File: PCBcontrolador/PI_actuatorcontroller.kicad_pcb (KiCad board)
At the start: 2 copper layers, 95.7 x 60 mm, 43 parts, among them IC1 TLV9032QDGKRQ1, J1 ACTUATOR1, J3 Barrel_Jack_Switch, U1 INA381A1IDSGR

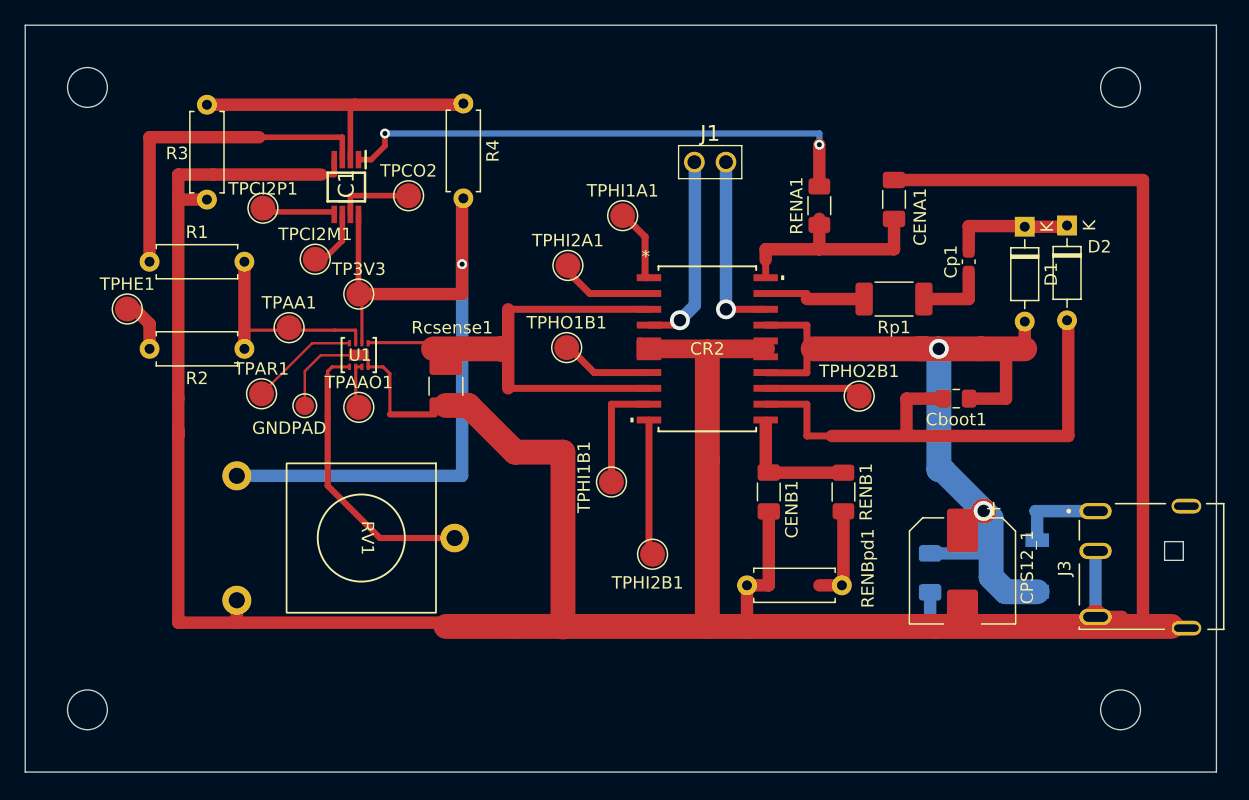
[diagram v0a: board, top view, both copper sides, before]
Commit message: PCB controller final version
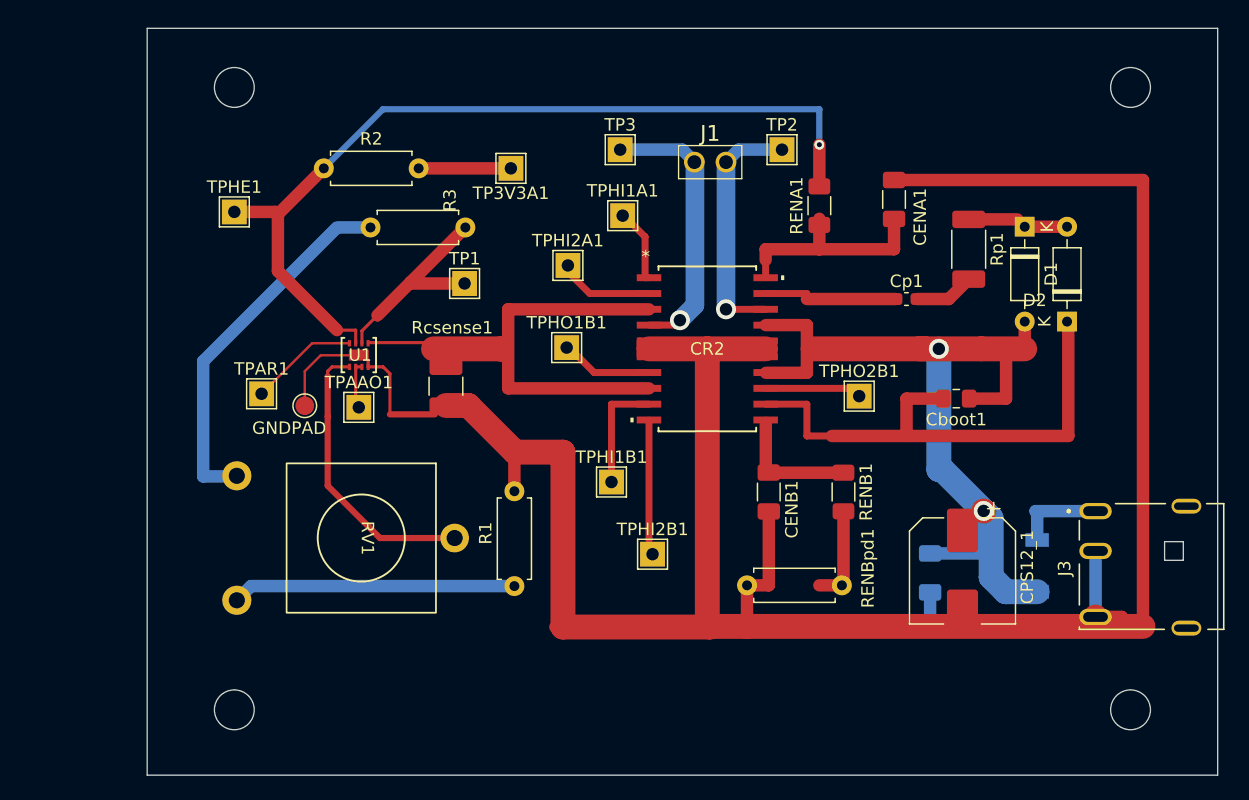
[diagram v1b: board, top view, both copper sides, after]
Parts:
- removed IC1: TLV9032QDGKRQ1, TLV9032QDGKRQ1:SOP65P490X110-8N
- removed R4: 2k, Resistor_THT:R_Axial_DIN0207_L6.3mm_D2.5mm_P7.62mm_Horizontal
- removed TP3V3, TPAA1, TPCI2M1, TPCI2P1, TPCO2: TestPoint, TestPoint:TestPoint_Pad_D2.0mm
- added TP1: TestPoint, TestPoint:TestPoint_THTPad_2.0x2.0mm_Drill1.0mm, F.Cu at (134.5, 81.8)
- added TP2: TestPoint, TestPoint:TestPoint_THTPad_2.0x2.0mm_Drill1.0mm, F.Cu at (160.0, 71.0)
- added TP3: TestPoint, TestPoint:TestPoint_THTPad_2.0x2.0mm_Drill1.0mm, F.Cu at (147.0, 71.0)
- added TP3V3A1: TestPoint, TestPoint:TestPoint_THTPad_2.0x2.0mm_Drill1.0mm, F.Cu at (138.2, 72.5)
- R1, R3: value 2k -> 10K
- R2: value 2k -> 10k
- TPAAO1, TPAR1, TPHE1, TPHI1A1, TPHI1B1, TPHI2A1, TPHI2B1, TPHO1B1, TPHO2B1: footprint TestPoint:TestPoint_Pad_D2.0mm -> TestPoint:TestPoint_THTPad_2.0x2.0mm_Drill1.0mm
- moved R1 39.2 mm to (138.5, 106.1), turned to 90 degrees
- moved R3 20.9 mm to (134.6, 77.2), turned to 180 degrees
- moved R2 15.8 mm to (123.2, 72.5), turned to 0 degrees
- moved REF** 11.8 mm to (116.0, 66.0)
- moved REF** 11.8 mm to (116.0, 115.9)
- moved TPHE1 11.6 mm to (116.0, 76.0)
- moved D2 7.72 mm to (182.9, 84.8), turned to 90 degrees
- moved Rp1 7.21 mm to (175.0, 79.0), turned to -90 degrees
- moved Cp1 5.83 mm to (170.0, 83.0), turned to 0 degrees
- moved REF** 0.80 mm to (188.0, 116.0)
- moved REF** 0.80 mm to (188.0, 66.0)
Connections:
- Cp1 pad 1: Net-(Cp1-Pad1) -> Net-(CR2-VCP)
- Cp1 pad 2: Net-(D1-K) -> Net-(Cp1-Pad2)
- D2 pad 1: Net-(D1-K) -> Net-(CR2-VBOOT)
- D2 pad 2: Net-(CR2-VBOOT) -> Net-(D1-K)
- GNDPAD pad 1: (no net) -> GND
- R1 pad 1: /EnA_soft -> Net-(R1-Pad1)
- R1 pad 2: /calert -> GND
- R2 pad 1: /calert -> /GPIO enable
- R2 pad 2: /GPIO enable -> Net-(R2-Pad2)
- R3 pad 1: GND -> +3V3
- R3 pad 2: Net-(IC1-IN1-) -> Net-(R3-Pad2)
- RENA1 pad 2: /EnA_buf -> /GPIO enable
- RV1 pad 1: +3V3 -> Net-(R3-Pad2)
- RV1 pad 3: GND -> Net-(R1-Pad1)
- Rp1 pad 1: Net-(Cp1-Pad1) -> Net-(D1-K)
- Rp1 pad 2: Net-(CR2-VCP) -> Net-(Cp1-Pad2)
- U1 pad 3: /calert -> /GPIO enable
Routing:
- net GND: track 309.0 -> 225.2 mm
- net /GPIO enable: track 3.98 -> 71.7 mm, vias 0 -> 1
- net +3V3: track 61.2 -> 17.6 mm, vias 1 -> 0
- net /EnA_buf: track 43.6 -> 0.00 mm, vias 2 -> 0
- net Net-(R3-Pad2): track 0.00 -> 29.3 mm
- net /EnA_soft: track 27.3 -> 0.00 mm
- net Net-(IC1-IN1-): track 25.2 -> 0.00 mm
- net Net-(R1-Pad1): track 0.00 -> 22.8 mm
- net /calert: track 17.0 -> 0.00 mm
- net Net-(R2-Pad2): track 0.00 -> 7.02 mm
- net Net-(CR2-OUT1A): track 15.9 -> 22.3 mm
- net Net-(Cp1-Pad1): track 5.74 -> 0.00 mm
- net Net-(IC1-OUT2): track 5.19 -> 0.00 mm
- net Net-(IC1-IN2+): track 5.03 -> 0.00 mm
- net Net-(CR2-OUT2A): track 15.0 -> 19.9 mm
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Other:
- board size 95.7 x 60 mm -> 86 x 60 mm
